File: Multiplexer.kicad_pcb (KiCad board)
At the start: 2 copper layers, 30 x 80 mm, 41 parts, among them J1 Conn_Coaxial, J2 Conn_Coaxial, J3 Conn_Coaxial, J4 Conn_Coaxial, J5 Conn_Coaxial

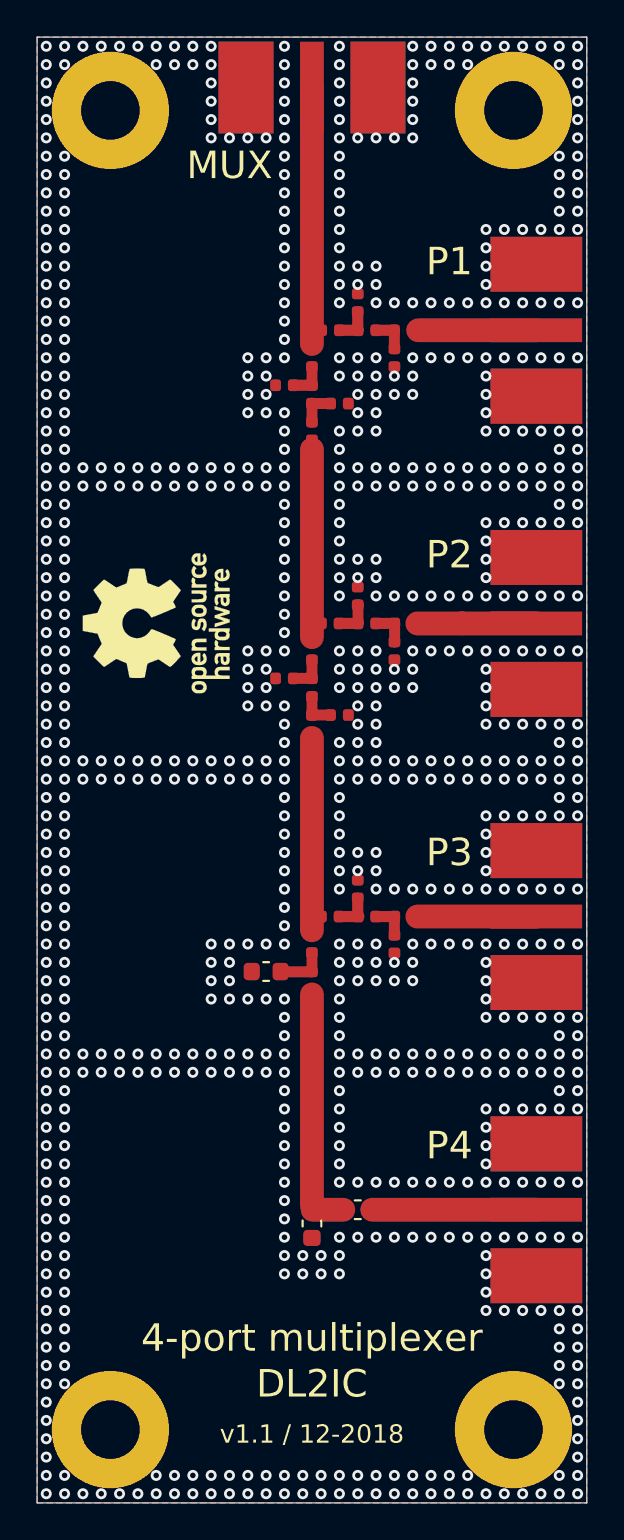
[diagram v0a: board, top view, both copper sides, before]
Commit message: Update
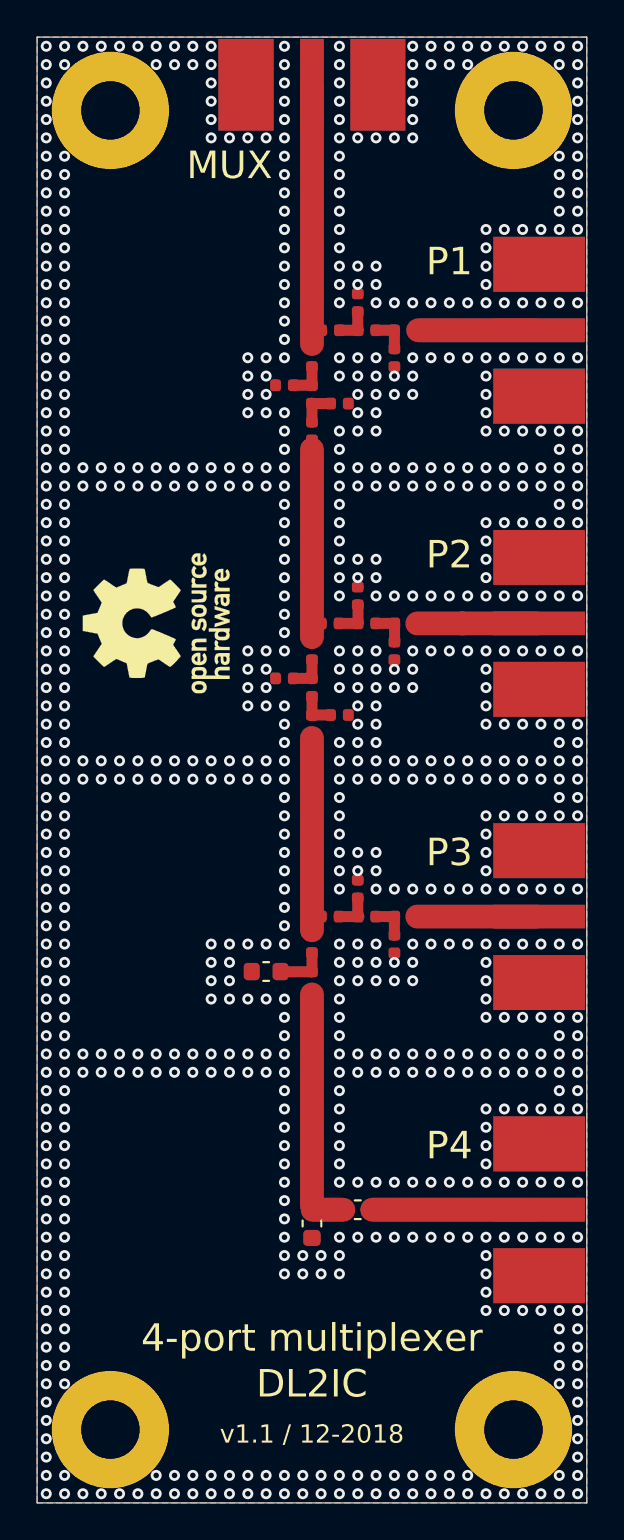
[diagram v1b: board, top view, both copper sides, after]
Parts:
- moved J1 0.15 mm to (115.0, 82.6)
- moved J2 0.15 mm to (127.4, 96.0)
- moved J3 0.15 mm to (127.4, 112.0)
- moved J4 0.15 mm to (127.4, 128.0)
- moved J5 0.15 mm to (127.4, 144.0)
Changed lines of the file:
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@@
       (drillshape 0)
       (scaleselection 1)
-      (outputdirectory "Multiplexer/"))
+      (outputdirectory "Multiplexer_gerber/"))
   )
   (net 0 "")
@@
   )
   (module Multiplexer:SMA_Connector (layer F.Cu)
-    (at 115 82.75)
+    (at 115 82.6)
     (fp_text reference J1 (at 0 3.6) (layer F.SilkS) hide
       (effects (font (size 1 1) (thickness 0.15)))
@@
   )
   (module Multiplexer:SMA_Connector (layer F.Cu)
-    (at 127.25 96 270)
+    (at 127.4 96 270)
     (fp_text reference J2 (at 0 6.8 270) (layer F.SilkS) hide
       (effects (font (size 1 1) (thickness 0.15)))
@@
   )
   (module Multiplexer:SMA_Connector (layer F.Cu)
-    (at 127.25 112 270)
+    (at 127.4 112 270)
     (fp_text reference J3 (at 0 6.8 270) (layer F.SilkS) hide
       (effects (font (size 1 1) (thickness 0.15)))
@@
   )
   (module Multiplexer:SMA_Connector (layer F.Cu)
-    (at 127.25 128 270)
+    (at 127.4 128 270)
     (fp_text reference J4 (at 0 6.8 270) (layer F.SilkS) hide
       (effects (font (size 1 1) (thickness 0.15)))
@@
   )
   (module Multiplexer:SMA_Connector (layer F.Cu)
-    (at 127.25 144 270)
+    (at 127.4 144 270)
     (fp_text reference J5 (at 0 6.8 270) (layer F.SilkS) hide
       (effects (font (size 1 1) (thickness 0.15)))
@@
   (gr_line (start 100 160) (end 130 160) (layer Edge.Cuts) (width 0.05))
   (gr_line (start 100 80) (end 100 160) (layer Edge.Cuts) (width 0.05))
+  (via (at 102.5 119.5) (size 0.6) (drill 0.3) (layers F.Cu B.Cu) (net 2))
+  (via (at 105.5 120.5) (size 0.6) (drill 0.3) (layers F.Cu B.Cu) (net 2))
+  (via (at 102.5 120.5) (size 0.6) (drill 0.3) (layers F.Cu B.Cu) (net 2))
+  (via (at 104.5 119.5) (size 0.6) (drill 0.3) (layers F.Cu B.Cu) (net 2))
+  (via (at 106.5 120.5) (size 0.6) (drill 0.3) (layers F.Cu B.Cu) (net 2))
+  (via (at 106.5 119.5) (size 0.6) (drill 0.3) (layers F.Cu B.Cu) (net 2))
+  (via (at 104.5 120.5) (size 0.6) (drill 0.3) (layers F.Cu B.Cu) (net 2))
+  (via (at 103.5 120.5) (size 0.6) (drill 0.3) (layers F.Cu B.Cu) (net 2))
+  (via (at 103.5 119.5) (size 0.6) (drill 0.3) (layers F.Cu B.Cu) (net 2))
+  (via (at 105.5 119.5) (size 0.6) (drill 0.3) (layers F.Cu B.Cu) (net 2))
+  (via (at 101.5 121.5) (size 0.6) (drill 0.3) (layers F.Cu B.Cu) (net 2))
+  (via (at 101.5 120.5) (size 0.6) (drill 0.3) (layers F.Cu B.Cu) (net 2))
+  (via (at 101.5 118.5) (size 0.6) (drill 0.3) (layers F.Cu B.Cu) (net 2))
+  (via (at 101.5 119.5) (size 0.6) (drill 0.3) (layers F.Cu B.Cu) (net 2))
   (segment (start 115 82.75) (end 115 96.75) (width 1.3) (layer F.Cu) (net 1))
   (via (at 113.5 105.5) (size 0.6) (drill 0.3) (layers F.Cu B.Cu) (net 2))
@@
   (via (at 100.5 107.5) (size 0.6) (drill 0.3) (layers F.Cu B.Cu) (net 2))
   (via (at 100.5 111.5) (size 0.6) (drill 0.3) (layers F.Cu B.Cu) (net 2))
-  (via (at 101.5 118.5) (size 0.6) (drill 0.3) (layers F.Cu B.Cu) (net 2))
-  (via (at 101.5 119.5) (size 0.6) (drill 0.3) (layers F.Cu B.Cu) (net 2))
   (via (at 100.5 115.5) (size 0.6) (drill 0.3) (layers F.Cu B.Cu) (net 2))
   (via (at 101.5 116.5) (size 0.6) (drill 0.3) (layers F.Cu B.Cu) (net 2))
@@
   (via (at 101.5 124.5) (size 0.6) (drill 0.3) (layers F.Cu B.Cu) (net 2))
   (via (at 101.5 125.5) (size 0.6) (drill 0.3) (layers F.Cu B.Cu) (net 2))
-  (via (at 101.5 120.5) (size 0.6) (drill 0.3) (layers F.Cu B.Cu) (net 2))
   (via (at 100.5 120.5) (size 0.6) (drill 0.3) (layers F.Cu B.Cu) (net 2))
   (via (at 101.5 129.5) (size 0.6) (drill 0.3) (layers F.Cu B.Cu) (net 2))
@@
   (via (at 101.5 126.5) (size 0.6) (drill 0.3) (layers F.Cu B.Cu) (net 2))
   (via (at 100.5 128.5) (size 0.6) (drill 0.3) (layers F.Cu B.Cu) (net 2))
-  (via (at 101.5 121.5) (size 0.6) (drill 0.3) (layers F.Cu B.Cu) (net 2))
   (via (at 100.5 124.5) (size 0.6) (drill 0.3) (layers F.Cu B.Cu) (net 2))
   (via (at 100.5 122.5) (size 0.6) (drill 0.3) (layers F.Cu B.Cu) (net 2))
@@
   (via (at 110.5 119.5) (size 0.6) (drill 0.3) (layers F.Cu B.Cu) (net 2))
   (via (at 113.5 119.5) (size 0.6) (drill 0.3) (layers F.Cu B.Cu) (net 2))
-  (via (at 106.5 119.5) (size 0.6) (drill 0.3) (layers F.Cu B.Cu) (net 2))
-  (via (at 106.5 120.5) (size 0.6) (drill 0.3) (layers F.Cu B.Cu) (net 2))
   (via (at 108.5 120.5) (size 0.6) (drill 0.3) (layers F.Cu B.Cu) (net 2))
-  (via (at 104.5 119.5) (size 0.6) (drill 0.3) (layers F.Cu B.Cu) (net 2))
-  (via (at 102.5 120.5) (size 0.6) (drill 0.3) (layers F.Cu B.Cu) (net 2))
-  (via (at 105.5 120.5) (size 0.6) (drill 0.3) (layers F.Cu B.Cu) (net 2))
   (via (at 108.5 119.5) (size 0.6) (drill 0.3) (layers F.Cu B.Cu) (net 2))
   (via (at 112.5 120.5) (size 0.6) (drill 0.3) (layers F.Cu B.Cu) (net 2))
   (via (at 112.5 119.5) (size 0.6) (drill 0.3) (layers F.Cu B.Cu) (net 2))
-  (via (at 102.5 119.5) (size 0.6) (drill 0.3) (layers F.Cu B.Cu) (net 2))
   (via (at 111.5 120.5) (size 0.6) (drill 0.3) (layers F.Cu B.Cu) (net 2))
   (via (at 110.5 120.5) (size 0.6) (drill 0.3) (layers F.Cu B.Cu) (net 2))
-  (via (at 105.5 119.5) (size 0.6) (drill 0.3) (layers F.Cu B.Cu) (net 2))
-  (via (at 103.5 119.5) (size 0.6) (drill 0.3) (layers F.Cu B.Cu) (net 2))
   (via (at 113.5 120.5) (size 0.6) (drill 0.3) (layers F.Cu B.Cu) (net 2))
   (via (at 109.5 119.5) (size 0.6) (drill 0.3) (layers F.Cu B.Cu) (net 2))
   (via (at 107.5 120.5) (size 0.6) (drill 0.3) (layers F.Cu B.Cu) (net 2))
-  (via (at 103.5 120.5) (size 0.6) (drill 0.3) (layers F.Cu B.Cu) (net 2))
   (via (at 111.5 119.5) (size 0.6) (drill 0.3) (layers F.Cu B.Cu) (net 2))
-  (via (at 104.5 120.5) (size 0.6) (drill 0.3) (layers F.Cu B.Cu) (net 2))
   (via (at 109.5 136.5) (size 0.6) (drill 0.3) (layers F.Cu B.Cu) (net 2))
   (via (at 107.5 135.5) (size 0.6) (drill 0.3) (layers F.Cu B.Cu) (net 2))
